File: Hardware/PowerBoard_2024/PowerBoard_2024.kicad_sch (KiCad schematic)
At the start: 218 parts, among them J1 RJ45_LED_Shielded, Q1 BSS138, Q10 BSS138, Q11 BSS138, Q12 IRF7606PBF, Q13 IRF7606PBF, Q14 SPD30P06PGBTMA1, Q15 BSS138, Q16 SPD30P06PGBTMA1, Q17 BSS138, Q18 BSS138, Q19 BSS138, Q2 IRF7606PBF, Q20 IRF7606PBF, Q21 IRF7606PBF, Q22 SPD30P06PGBTMA1, Q23 BSS138, Q24 SPD30P06PGBTMA1, Q25 BSS138, Q26 SPD30P06PGBTMA1, Q27 BSS138, Q28 SPD30P06PGBTMA1, Q29 BSS138, Q3 BSS138, Q30 SPD30P06PGBTMA1, Q4 IRF7606PBF, Q5 BSS138, Q6 SPD30P06PGBTMA1, Q7 BSS138, Q8 SPD30P06PGBTMA1, Q9 BSS138, U1 3V3, U10 ACS725xLCTR-20AB, U11 ACS725xLCTR-20AB, U12 ACS725xLCTR-20AB, U13 ACS725xLCTR-20AB, U14 ACS725xLCTR-20AB, U15 Teensy4.1_DEV-16771, U16 ACS725xLCTR-20AB, U17 ACS725xLCTR-20AB, U18 ACS725xLCTR-20AB, U19 ACS725xLCTR-20AB, U2 ACS725xLCTR-20AB, U20 PKE3316ZPI, U21 ACS725xLCTR-20AB, U22 PKE3316ZPI, U23 ACS725xLCTR-20AB, U3 ACS725xLCTR-20AB, U4 ACS725xLCTR-20AB, U5 ACS725xLCTR-20AB, U6 ACS725xLCTR-20AB, U7 ACS725xLCTR-20AB, U8 ACS725xLCTR-20AB, U9 ACS725xLCTR-20AB

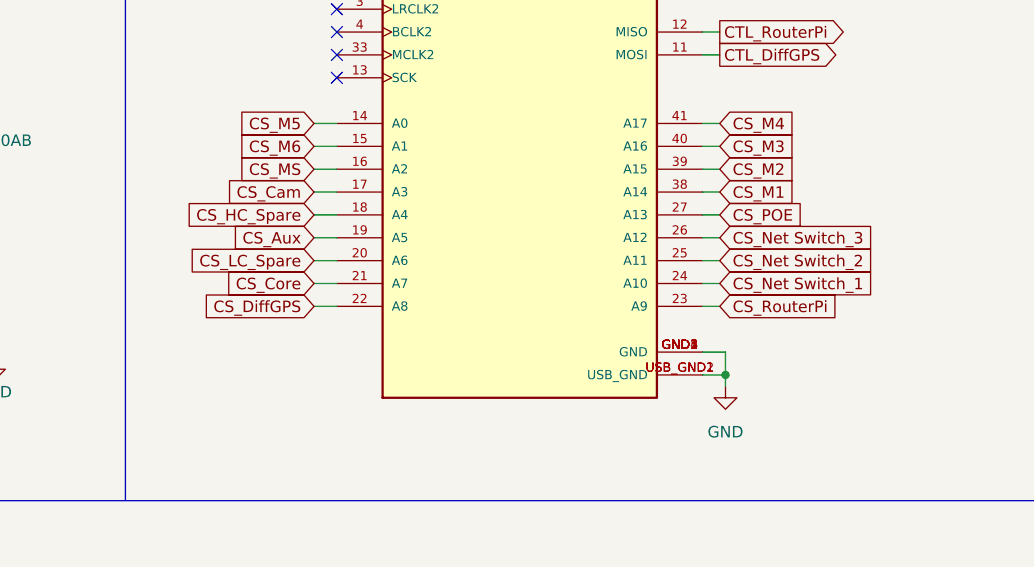
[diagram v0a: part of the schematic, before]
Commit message: Layout Review Ready
Made the traces pretty
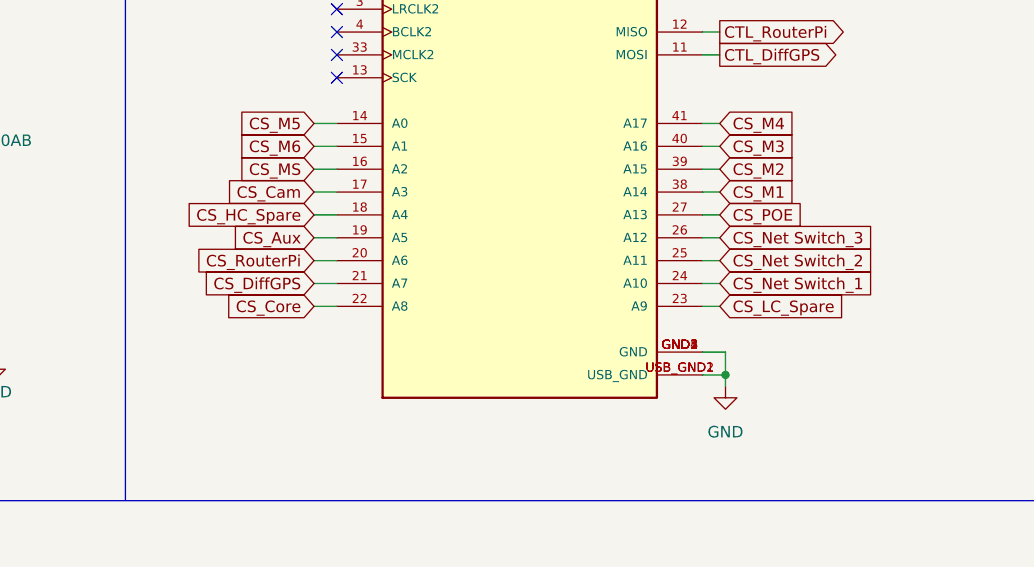
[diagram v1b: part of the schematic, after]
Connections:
- net CS_Core: now also U15.22 (A8); no longer U15.21 (A7)
- net CS_DiffGPS: now also U15.21 (A7); no longer U15.22 (A8)
- net CS_LC_Spare: now also U15.23 (A9); no longer U15.20 (A6)
- net CS_RouterPi: now also U15.20 (A6); no longer U15.23 (A9)
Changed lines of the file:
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@@
     (stroke (width 0) (type default))
   )
+  (wire (pts (xy 471.17 255.905) (xy 473.71 255.905))
+    (stroke (width 0) (type default))
+  )
   (wire (pts (xy 403.225 117.475) (xy 403.225 121.285))
     (stroke (width 0) (type default))
@@
     (stroke (width 0) (type default))
   )
+  (wire (pts (xy 514.35 258.445) (xy 516.255 258.445))
+    (stroke (width 0) (type default))
+  )
   (wire (pts (xy 562.61 111.125) (xy 562.61 105.41))
     (stroke (width 0) (type default))
@@
     (stroke (width 0) (type default))
   )
-  (wire (pts (xy 471.17 255.905) (xy 473.71 255.905))
-    (stroke (width 0) (type default))
-  )
   (wire (pts (xy 375.285 64.135) (xy 375.285 67.945))
     (stroke (width 0) (type default))
@@
     (stroke (width 0) (type default))
   )
+  (wire (pts (xy 471.17 253.365) (xy 473.71 253.365))
+    (stroke (width 0) (type default))
+  )
   (wire (pts (xy 322.58 36.195) (xy 322.58 34.29))
     (stroke (width 0) (type default))
@@
     (stroke (width 0) (type default))
   )
-  (wire (pts (xy 471.17 253.365) (xy 473.71 253.365))
-    (stroke (width 0) (type default))
-  )
   (wire (pts (xy 202.565 39.37) (xy 210.82 39.37))
     (stroke (width 0) (type default))
@@
     (stroke (width 0) (type default))
   )
-  (wire (pts (xy 514.35 258.445) (xy 516.255 258.445))
-    (stroke (width 0) (type default))
-  )
   (wire (pts (xy 361.315 118.745) (xy 361.315 121.285))
     (stroke (width 0) (type default))
@@
     (stroke (width 0) (type default))
   )
-  (wire (pts (xy 471.17 258.445) (xy 473.71 258.445))
-    (stroke (width 0) (type default))
-  )
   (wire (pts (xy 389.89 67.945) (xy 400.05 67.945))
     (stroke (width 0) (type default))
@@
     (stroke (width 0) (type default))
   )
+  (wire (pts (xy 471.17 258.445) (xy 473.71 258.445))
+    (stroke (width 0) (type default))
+  )
   (wire (pts (xy 154.305 187.325) (xy 154.305 189.865))
     (stroke (width 0) (type default))
@@
     )
   )
-  (global_label "CS_Core" (shape input) (at 471.17 255.905 180) (fields_autoplaced)
+  (global_label "CS_Core" (shape input) (at 471.17 258.445 180) (fields_autoplaced)
     (effects (font (size 1.27 1.27)) (justify right))
-    (property "Intersheetrefs" "${INTERSHEET_REFS}" (at 460.4439 255.905 0)
+    (property "Intersheetrefs" "${INTERSHEET_REFS}" (at 460.4439 258.445 0)
       (effects (font (size 1.27 1.27)) (justify right) hide)
     )
@@
     )
   )
-  (global_label "CS_RouterPi" (shape input) (at 516.255 258.445 0) (fields_autoplaced)
-    (effects (font (size 1.27 1.27)) (justify left))
-    (property "Intersheetrefs" "${INTERSHEET_REFS}" (at 530.7306 258.445 0)
-      (effects (font (size 1.27 1.27)) (justify left) hide)
+  (global_label "CS_RouterPi" (shape input) (at 471.17 253.365 180) (fields_autoplaced)
+    (effects (font (size 1.27 1.27)) (justify right))
+    (property "Intersheetrefs" "${INTERSHEET_REFS}" (at 456.6944 253.365 0)
+      (effects (font (size 1.27 1.27)) (justify right) hide)
     )
   )
@@
     )
   )
-  (global_label "CS_DiffGPS" (shape input) (at 471.17 258.445 180) (fields_autoplaced)
+  (global_label "CS_DiffGPS" (shape input) (at 471.17 255.905 180) (fields_autoplaced)
     (effects (font (size 1.27 1.27)) (justify right))
-    (property "Intersheetrefs" "${INTERSHEET_REFS}" (at 457.662 258.445 0)
+    (property "Intersheetrefs" "${INTERSHEET_REFS}" (at 457.662 255.905 0)
       (effects (font (size 1.27 1.27)) (justify right) hide)
     )
@@
     )
   )
-  (global_label "CS_LC_Spare" (shape input) (at 471.17 253.365 180) (fields_autoplaced)
-    (effects (font (size 1.27 1.27)) (justify right))
-    (property "Intersheetrefs" "${INTERSHEET_REFS}" (at 456.0897 253.365 0)
-      (effects (font (size 1.27 1.27)) (justify right) hide)
+  (global_label "CS_LC_Spare" (shape input) (at 516.255 258.445 0) (fields_autoplaced)
+    (effects (font (size 1.27 1.27)) (justify left))
+    (property "Intersheetrefs" "${INTERSHEET_REFS}" (at 531.3353 258.445 0)
+      (effects (font (size 1.27 1.27)) (justify left) hide)
     )
   )

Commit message: Fixed planes
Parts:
- U10, U11, U18, U19, U2, U3, U6, U7: footprint Package_SO:SOIC-8_3.9x4.9mm_P1.27mm -> Package_SO:SOP-8_3.9x4.9mm_P1.27mm
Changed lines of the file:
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@@
       (effects (font (size 1.27 1.27)) (justify left))
     )
-    (property "Footprint" "Package_SO:SOIC-8_3.9x4.9mm_P1.27mm" (at 252.73 198.12 0)
+    (property "Footprint" "Package_SO:SOP-8_3.9x4.9mm_P1.27mm" (at 252.73 198.12 0)
       (effects (font (size 1.27 1.27) italic) (justify left) hide)
     )
@@
       (effects (font (size 1.27 1.27)) (justify left))
     )
-    (property "Footprint" "Package_SO:SOIC-8_3.9x4.9mm_P1.27mm" (at 347.345 203.2 0)
+    (property "Footprint" "Package_SO:SOP-8_3.9x4.9mm_P1.27mm" (at 347.345 203.2 0)
       (effects (font (size 1.27 1.27) italic) (justify left) hide)
     )
@@
       (effects (font (size 1.27 1.27)) (justify left))
     )
-    (property "Footprint" "Package_SO:SOIC-8_3.9x4.9mm_P1.27mm" (at 415.925 202.565 0)
+    (property "Footprint" "Package_SO:SOP-8_3.9x4.9mm_P1.27mm" (at 415.925 202.565 0)
       (effects (font (size 1.27 1.27) italic) (justify left) hide)
     )
@@
       (effects (font (size 1.27 1.27)) (justify left))
     )
-    (property "Footprint" "Package_SO:SOIC-8_3.9x4.9mm_P1.27mm" (at 217.17 250.825 0)
+    (property "Footprint" "Package_SO:SOP-8_3.9x4.9mm_P1.27mm" (at 217.17 250.825 0)
       (effects (font (size 1.27 1.27) italic) (justify left) hide)
     )
@@
       (effects (font (size 1.27 1.27)) (justify left))
     )
-    (property "Footprint" "Package_SO:SOIC-8_3.9x4.9mm_P1.27mm" (at 415.925 254 0)
+    (property "Footprint" "Package_SO:SOP-8_3.9x4.9mm_P1.27mm" (at 415.925 254 0)
       (effects (font (size 1.27 1.27) italic) (justify left) hide)
     )
@@
       (effects (font (size 1.27 1.27)) (justify left))
     )
-    (property "Footprint" "Package_SO:SOIC-8_3.9x4.9mm_P1.27mm" (at 348.615 254 0)
+    (property "Footprint" "Package_SO:SOP-8_3.9x4.9mm_P1.27mm" (at 348.615 254 0)
       (effects (font (size 1.27 1.27) italic) (justify left) hide)
     )
@@
       (effects (font (size 1.27 1.27)) (justify left))
     )
-    (property "Footprint" "Package_SO:SOIC-8_3.9x4.9mm_P1.27mm" (at 171.45 250.825 0)
+    (property "Footprint" "Package_SO:SOP-8_3.9x4.9mm_P1.27mm" (at 171.45 250.825 0)
       (effects (font (size 1.27 1.27) italic) (justify left) hide)
     )
@@
       (effects (font (size 1.27 1.27)) (justify left))
     )
-    (property "Footprint" "Package_SO:SOIC-8_3.9x4.9mm_P1.27mm" (at 182.88 197.485 0)
+    (property "Footprint" "Package_SO:SOP-8_3.9x4.9mm_P1.27mm" (at 182.88 197.485 0)
       (effects (font (size 1.27 1.27) italic) (justify left) hide)
     )
